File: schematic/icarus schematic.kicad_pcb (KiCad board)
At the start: 2 copper layers, 2 parts, among them U1 ESP32-S3, U2 BMI088

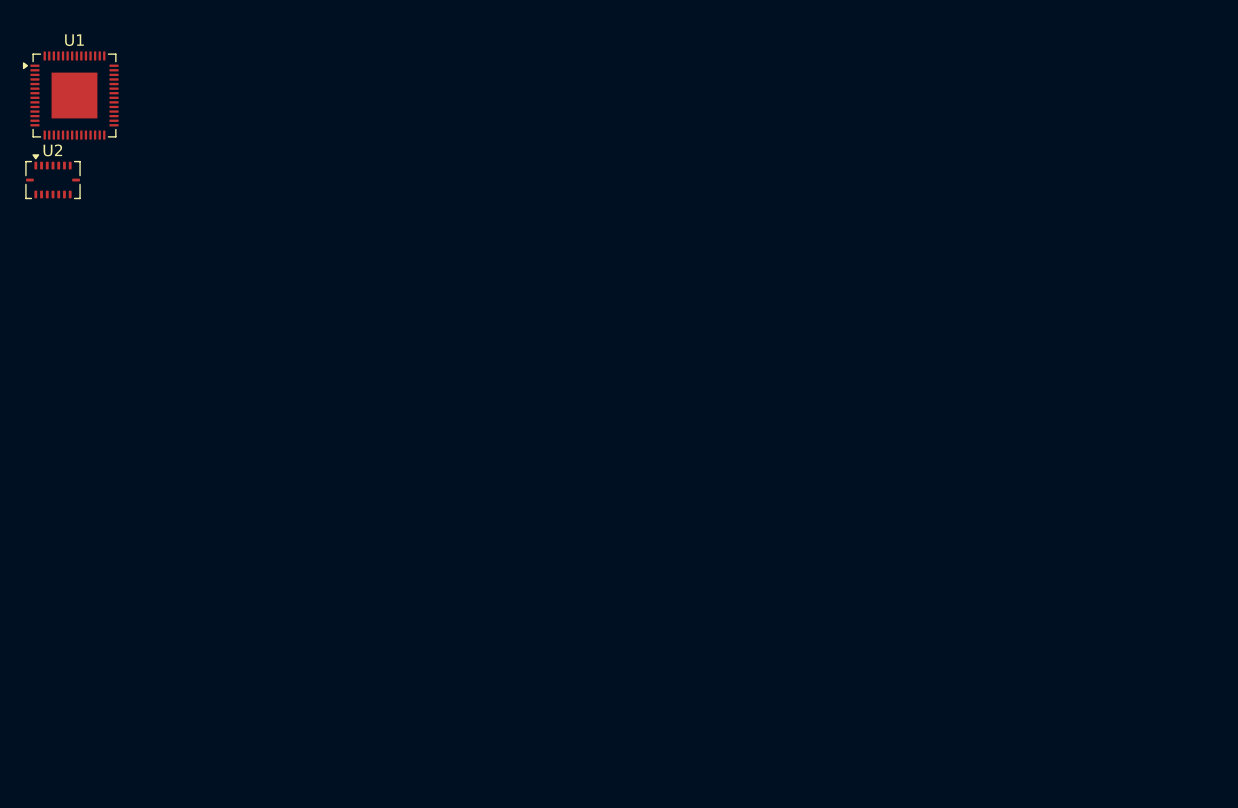
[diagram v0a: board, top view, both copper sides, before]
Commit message: added datasheets
other Datasheets

Added capacitors across motors

Added connectors instead of motors.

Add link to mini 100 brushed frame model

Remove URL from Frame file

Update Frame

Delete Frame

Add files via upload

this is the version -1 drone frame

PCB first iteration.
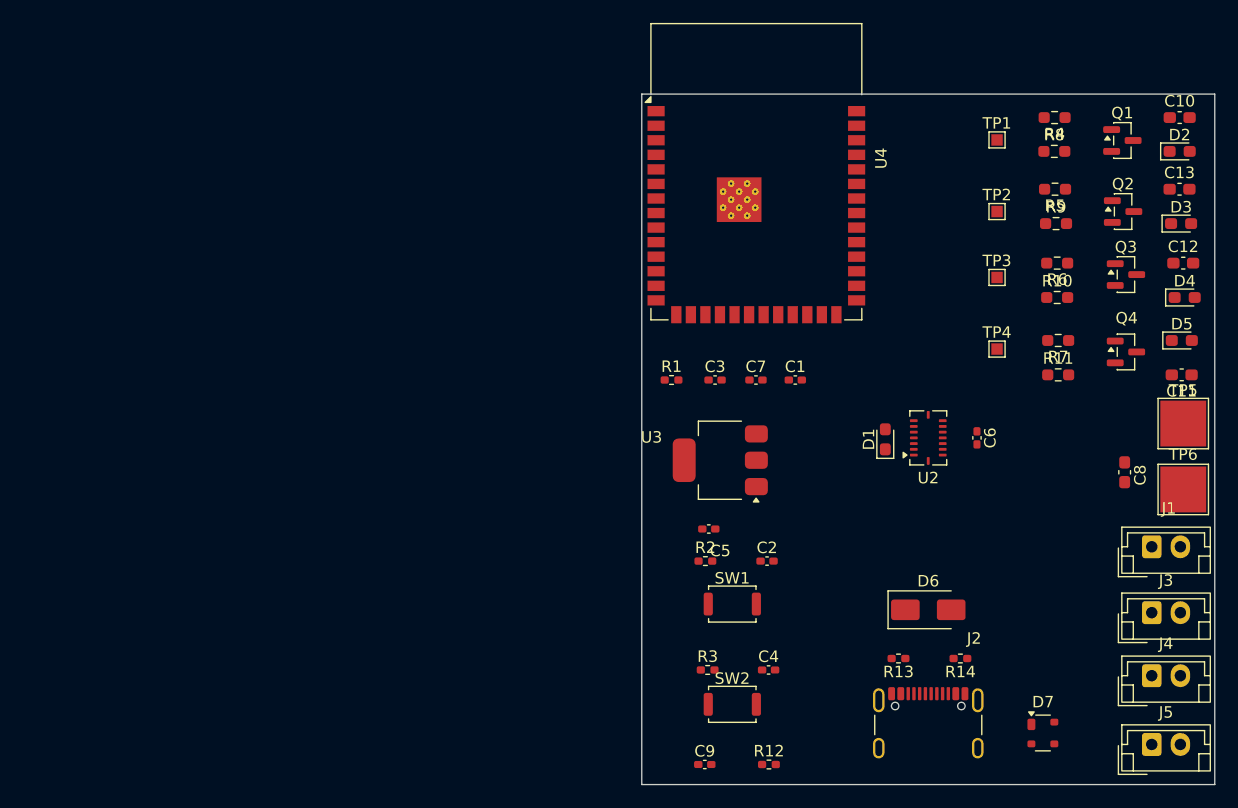
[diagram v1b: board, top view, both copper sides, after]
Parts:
- removed U1: ESP32-S3, Package_DFN_QFN:QFN-56-1EP_7x7mm_P0.4mm_EP4x4mm
- added C1: 10uF, Capacitor_SMD:C_0402_1005Metric_Pad0.74x0.62mm_HandSolder, F.Cu at (186.4, 96.0)
- added C10: 0.1uF, Capacitor_SMD:C_0603_1608Metric_Pad1.08x0.95mm_HandSolder, F.Cu at (219.9, 73.0)
- added C11: 0.1uF, Capacitor_SMD:C_0603_1608Metric_Pad1.08x0.95mm_HandSolder, F.Cu at (220.1, 95.5)
- added C12: 0.1uF, Capacitor_SMD:C_0603_1608Metric_Pad1.08x0.95mm_HandSolder, F.Cu at (220.2, 85.8)
- added C13: 0.1uF, Capacitor_SMD:C_0603_1608Metric_Pad1.08x0.95mm_HandSolder, F.Cu at (219.9, 79.3)
- added C2: 0.1uF, Capacitor_SMD:C_0402_1005Metric_Pad0.74x0.62mm_HandSolder, F.Cu at (183.9, 111.8)
- added C3: 10uF, Capacitor_SMD:C_0402_1005Metric_Pad0.74x0.62mm_HandSolder, F.Cu at (179.4, 96.0)
- added C4: 0.1uF, Capacitor_SMD:C_0402_1005Metric_Pad0.74x0.62mm_HandSolder, F.Cu at (184.1, 121.2)
- added C5: 100nf, Capacitor_SMD:C_0402_1005Metric_Pad0.74x0.62mm_HandSolder, F.Cu at (178.8, 109.0)
- added C6: 100nf, Capacitor_SMD:C_0402_1005Metric_Pad0.74x0.62mm_HandSolder, F.Cu at (202.2, 101.0)
- added C7: 100nf, Capacitor_SMD:C_0402_1005Metric_Pad0.74x0.62mm_HandSolder, F.Cu at (183.0, 96.0)
- added C8: 470uF, Capacitor_SMD:C_0603_1608Metric_Pad1.08x0.95mm_HandSolder, F.Cu at (215.1, 104.0)
- added C9: 100nf, Capacitor_SMD:C_0402_1005Metric_Pad0.74x0.62mm_HandSolder, F.Cu at (178.5, 129.5)
- added D1: LED, LED_SMD:LED_0603_1608Metric_Pad1.05x0.95mm_HandSolder, F.Cu at (194.2, 101.1)
- added D2: 1N5819, Diode_SMD:D_0603_1608Metric_Pad1.05x0.95mm_HandSolder, F.Cu at (219.9, 76.0)
- added D3: 1N5819, Diode_SMD:D_0603_1608Metric_Pad1.05x0.95mm_HandSolder, F.Cu at (220.1, 82.3)
- added D4: 1N5819, Diode_SMD:D_0603_1608Metric_Pad1.05x0.95mm_HandSolder, F.Cu at (220.4, 88.8)
- added D5: 1N5819, Diode_SMD:D_0603_1608Metric_Pad1.05x0.95mm_HandSolder, F.Cu at (220.1, 92.5)
- added D6: SS14, Diode_SMD:D_SMA, F.Cu at (198.0, 116.0)
- added D7: SP0503BAHT, Package_TO_SOT_SMD:SOT-143, F.Cu at (208.0, 126.8)
- added J1: Conn_01x02_Socket, Connector_JST:JST_EH_B2B-EH-A_1x02_P2.50mm_Vertical, F.Cu at (217.5, 110.5)
- added J2: USB_C_Receptacle_USB2.0_16P, Connector_USB:USB_C_Receptacle_GCT_USB4105-xx-A_16P_TopMnt_Horizontal, F.Cu at (198.0, 127.0)
- added J3: Conn_01x02_Socket, Connector_JST:JST_EH_B2B-EH-A_1x02_P2.50mm_Vertical, F.Cu at (217.5, 116.2)
- added J4: Conn_01x02_Socket, Connector_JST:JST_EH_B2B-EH-A_1x02_P2.50mm_Vertical, F.Cu at (217.5, 121.8)
- added J5: Conn_01x02_Socket, Connector_JST:JST_EH_B2B-EH-A_1x02_P2.50mm_Vertical, F.Cu at (217.5, 127.8)
- added Q1: AO3400A, Package_TO_SOT_SMD:SOT-23, F.Cu at (214.9, 75.0)
- added Q2: AO3400A, Package_TO_SOT_SMD:SOT-23, F.Cu at (215.0, 81.2)
- added Q3: AO3400A, Package_TO_SOT_SMD:SOT-23, F.Cu at (215.2, 86.8)
- added Q4: AO3400A, Package_TO_SOT_SMD:SOT-23, F.Cu at (215.2, 93.5)
- added R1: 220ohm, Resistor_SMD:R_0402_1005Metric_Pad0.72x0.64mm_HandSolder, F.Cu at (175.6, 96.0)
- added R10: 10k, Resistor_SMD:R_0603_1608Metric_Pad0.98x0.95mm_HandSolder, F.Cu at (209.2, 88.8)
- added R11: 10k, Resistor_SMD:R_0603_1608Metric_Pad0.98x0.95mm_HandSolder, F.Cu at (209.3, 95.5)
- added R12: 10k, Resistor_SMD:R_0402_1005Metric_Pad0.72x0.64mm_HandSolder, F.Cu at (184.1, 129.5)
- added R13: 5.1k, Resistor_SMD:R_0402_1005Metric_Pad0.72x0.64mm_HandSolder, F.Cu at (195.4, 120.2)
- added R14: 5.1k, Resistor_SMD:R_0402_1005Metric_Pad0.72x0.64mm_HandSolder, F.Cu at (200.8, 120.2)
- added R2: 10k, Resistor_SMD:R_0402_1005Metric_Pad0.72x0.64mm_HandSolder, F.Cu at (178.6, 111.8)
- added R3: 10k, Resistor_SMD:R_0402_1005Metric_Pad0.72x0.64mm_HandSolder, F.Cu at (178.8, 121.2)
- added R4: 100, Resistor_SMD:R_0603_1608Metric_Pad0.98x0.95mm_HandSolder, F.Cu at (209.0, 73.0)
- added R5: 100, Resistor_SMD:R_0603_1608Metric_Pad0.98x0.95mm_HandSolder, F.Cu at (209.1, 79.3)
- added R6: 100, Resistor_SMD:R_0603_1608Metric_Pad0.98x0.95mm_HandSolder, F.Cu at (209.2, 85.8)
- added R7: 100, Resistor_SMD:R_0603_1608Metric_Pad0.98x0.95mm_HandSolder, F.Cu at (209.3, 92.5)
- added R8: 10k, Resistor_SMD:R_0603_1608Metric_Pad0.98x0.95mm_HandSolder, F.Cu at (209.0, 76.0)
- added R9: 10k, Resistor_SMD:R_0603_1608Metric_Pad0.98x0.95mm_HandSolder, F.Cu at (209.2, 82.3)
- added SW1: SW_Push(BOOt), Button_Switch_SMD:SW_Push_SPST_NO_Alps_SKRK, F.Cu at (180.9, 115.5)
- added SW2: SW_Push(EN), Button_Switch_SMD:SW_Push_SPST_NO_Alps_SKRK, F.Cu at (180.9, 124.2)
- added TP1: TestPoint, TestPoint:TestPoint_Pad_1.0x1.0mm, F.Cu at (204.0, 75.0)
- added TP2: TestPoint, TestPoint:TestPoint_Pad_1.0x1.0mm, F.Cu at (204.0, 81.2)
- added TP3: TestPoint, TestPoint:TestPoint_Pad_1.0x1.0mm, F.Cu at (204.0, 87.0)
- added TP4: TestPoint, TestPoint:TestPoint_Pad_1.0x1.0mm, F.Cu at (204.0, 93.2)
- added TP5: TestPoint, TestPoint:TestPoint_Pad_4.0x4.0mm, F.Cu at (220.2, 99.8)
- added TP6: TestPoint, TestPoint:TestPoint_Pad_4.0x4.0mm, F.Cu at (220.2, 105.5)
- added U3: AMS1117-3.3, Package_TO_SOT_SMD:SOT-223-3_TabPin2, F.Cu at (179.8, 103.0)
- added U4: ESP32-S3-WROOM-1, RF_Module:ESP32-S3-WROOM-1, F.Cu at (183.0, 77.8)
- moved U2 79.6 mm to (198.0, 101.0), turned to 90 degrees
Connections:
- U2 pad 10: unconnected-(U2-SDO2-Pad10) -> /SD02
- U2 pad 11: unconnected-(U2-VDDIO-Pad11) -> /3.3V
- U2 pad 12: unconnected-(U2-INT3-Pad12) -> /INT3
- U2 pad 14: unconnected-(U2-~{CSB1}-Pad14) -> /CSB1
- U2 pad 15: unconnected-(U2-SDO1-Pad15) -> /SD01
- U2 pad 16: unconnected-(U2-INT1-Pad16) -> /INT1
- U2 pad 2: Net-(U2-GNDA-Pad2) -> GND
- U2 pad 3: unconnected-(U2-VDD-Pad3) -> /3.3V
- U2 pad 4: Net-(U2-GNDA-Pad2) -> GND
- U2 pad 5: unconnected-(U2-~{CSB2}-Pad5) -> /CSB2
- U2 pad 6: unconnected-(U2-GNDIO-Pad6) -> GND
- U2 pad 7: unconnected-(U2-PS-Pad7) -> GND
- U2 pad 8: unconnected-(U2-SCK/SCL-Pad8) -> /SCK
- U2 pad 9: unconnected-(U2-SDI/SDA-Pad9) -> /SDI
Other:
- board outline added: 50 x 60.2 mm
- board text added: "J2"
